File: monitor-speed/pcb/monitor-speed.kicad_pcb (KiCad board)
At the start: 2 copper layers, 60 x 70 mm, 0 parts

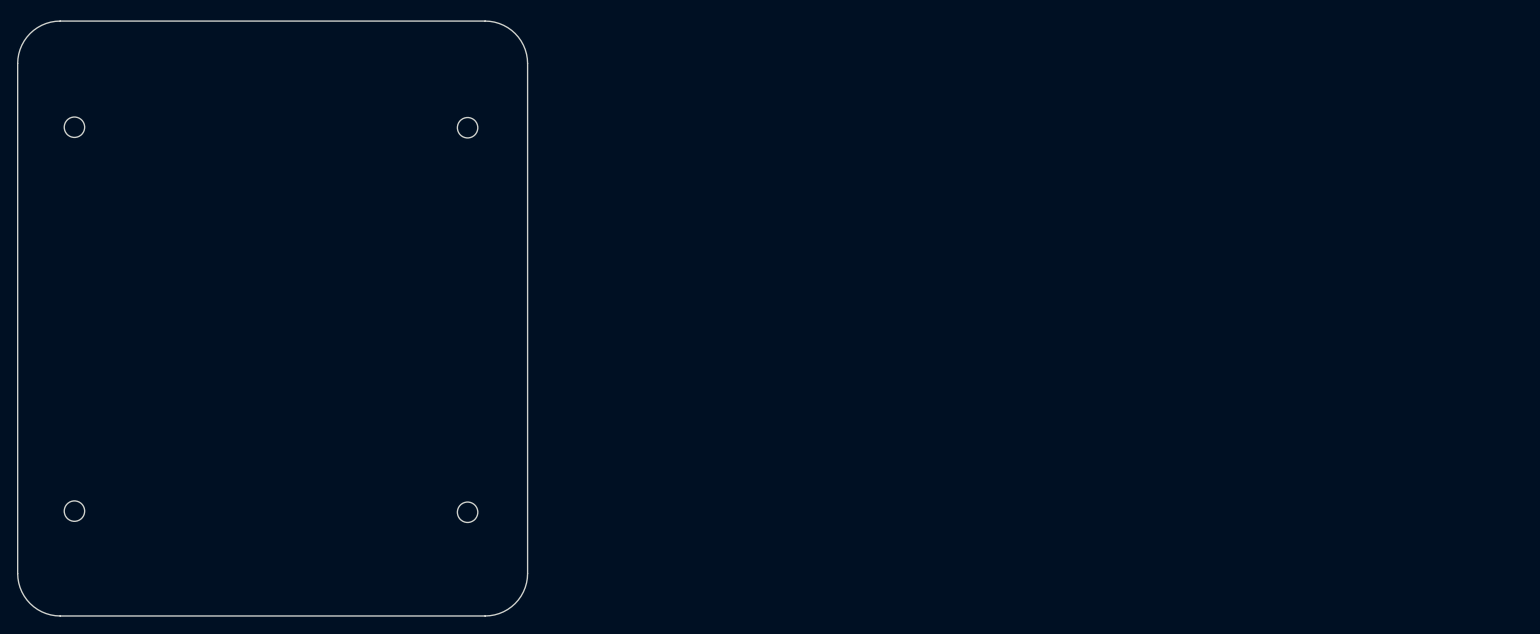
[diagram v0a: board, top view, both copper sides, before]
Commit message: Agregue capas interiores....
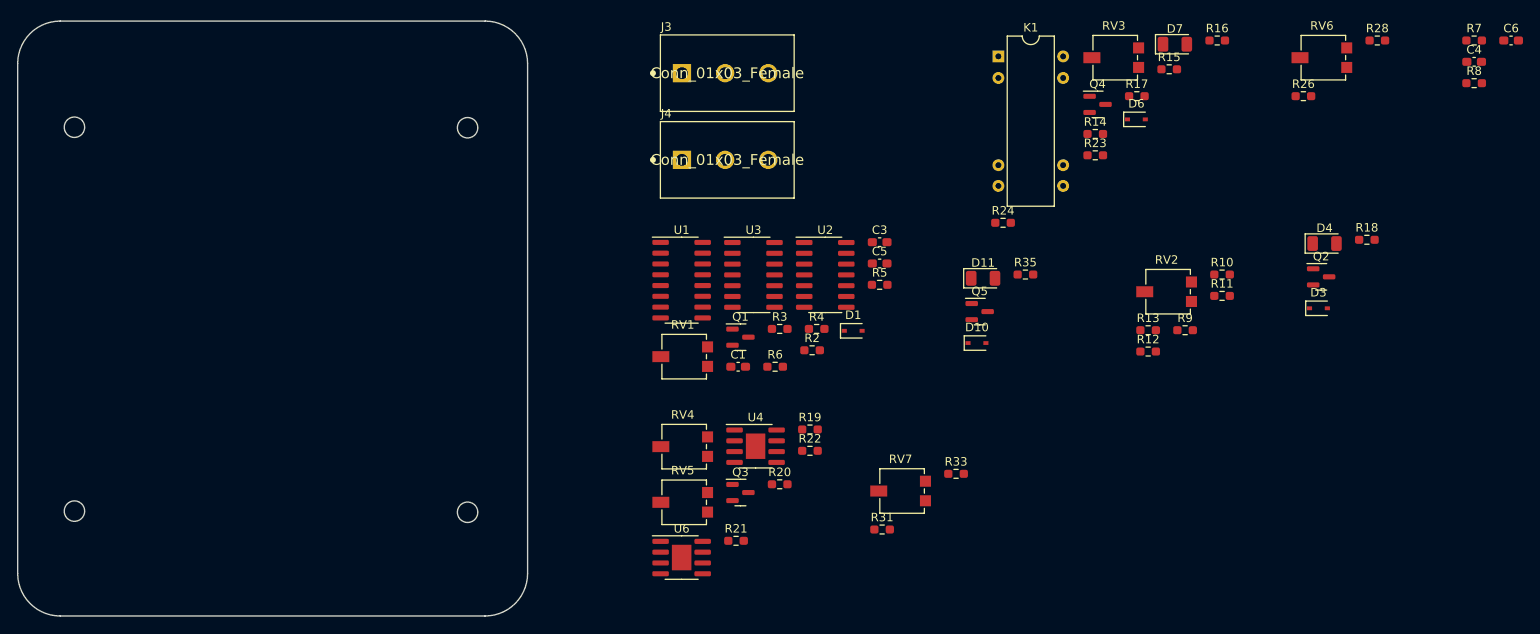
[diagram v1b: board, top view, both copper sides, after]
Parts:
- added C1: 100nF, Capacitor_SMD:C_0603_1608Metric_Pad1.08x0.95mm_HandSolder, F.Cu at (134.8, -93.3)
- added C3: 0.022uF, Capacitor_SMD:C_0603_1608Metric_Pad1.08x0.95mm_HandSolder, F.Cu at (151.4, -108.0)
- added C4: 1uF, Capacitor_SMD:C_0603_1608Metric_Pad1.08x0.95mm_HandSolder, F.Cu at (221.4, -129.2)
- added C5: 100nF, Capacitor_SMD:C_0603_1608Metric_Pad1.08x0.95mm_HandSolder, F.Cu at (151.4, -105.5)
- added C6: 1uF, Capacitor_SMD:C_0603_1608Metric_Pad1.08x0.95mm_HandSolder, F.Cu at (225.7, -131.7)
- added D1: 1N4148, Diode_SMD:D_SOD-323, F.Cu at (148.3, -97.6)
- added D10: 1N4148, Diode_SMD:D_SOD-323, F.Cu at (162.9, -96.1)
- added D11: RED, LED_SMD:LED_1206_3216Metric, F.Cu at (163.6, -103.7)
- added D3: 1N4148, Diode_SMD:D_SOD-323, F.Cu at (203.1, -100.2)
- added D4: RED, LED_SMD:LED_1206_3216Metric, F.Cu at (203.8, -107.8)
- added D6: 1N4148, Diode_SMD:D_SOD-323, F.Cu at (181.6, -122.4)
- added D7: LED, LED_SMD:LED_1206_3216Metric, F.Cu at (186.2, -131.3)
- added J3: Conn_01x03_Female, eec:TE-282841-3-0, F.Cu at (133.5, -127.9)
- added J4: Conn_01x03_Female, eec:TE-282841-3-0, F.Cu at (133.5, -117.7)
- added K1: DIPxx-1Cxx-51x, Relay_THT:Relay_StandexMeder_DIP_LowProfile, F.Cu at (165.4, -129.8)
- added Q1: BC848, Package_TO_SOT_SMD:SOT-23, F.Cu at (135.0, -96.8)
- added Q2: BC848, Package_TO_SOT_SMD:SOT-23, F.Cu at (203.4, -103.9)
- added Q3: PN2222A, Package_TO_SOT_SMD:SOT-23, F.Cu at (135.0, -78.5)
- added Q4: BC848, Package_TO_SOT_SMD:SOT-23, F.Cu at (177.1, -124.2)
- added Q5: BC848, Package_TO_SOT_SMD:SOT-23, F.Cu at (163.2, -99.8)
- added R10: 10M, Resistor_SMD:R_0603_1608Metric_Pad0.98x0.95mm_HandSolder, F.Cu at (191.7, -104.2)
- added R11: 47K, Resistor_SMD:R_0603_1608Metric_Pad0.98x0.95mm_HandSolder, F.Cu at (191.7, -101.7)
- added R12: 68K, Resistor_SMD:R_0603_1608Metric_Pad0.98x0.95mm_HandSolder, F.Cu at (183.0, -95.1)
- added R13: 1k, Resistor_SMD:R_0603_1608Metric_Pad0.98x0.95mm_HandSolder, F.Cu at (183.0, -97.6)
- added R14: 47K, Resistor_SMD:R_0603_1608Metric_Pad0.98x0.95mm_HandSolder, F.Cu at (176.8, -120.7)
- added R15: 10K, Resistor_SMD:R_0603_1608Metric_Pad0.98x0.95mm_HandSolder, F.Cu at (185.5, -128.3)
- added R16: 68K, Resistor_SMD:R_0603_1608Metric_Pad0.98x0.95mm_HandSolder, F.Cu at (191.1, -131.7)
- added R17: 10M, Resistor_SMD:R_0603_1608Metric_Pad0.98x0.95mm_HandSolder, F.Cu at (181.7, -125.2)
- added R18: 6.8K, Resistor_SMD:R_0603_1608Metric_Pad0.98x0.95mm_HandSolder, F.Cu at (208.8, -108.3)
- added R19: 10k, Resistor_SMD:R_0603_1608Metric_Pad0.98x0.95mm_HandSolder, F.Cu at (143.2, -85.9)
- added R2: 100K, Resistor_SMD:R_0603_1608Metric_Pad0.98x0.95mm_HandSolder, F.Cu at (143.5, -95.3)
- added R20: 100k, Resistor_SMD:R_0603_1608Metric_Pad0.98x0.95mm_HandSolder, F.Cu at (139.7, -79.5)
- added R21: 1k, Resistor_SMD:R_0603_1608Metric_Pad0.98x0.95mm_HandSolder, F.Cu at (134.5, -72.8)
- added R22: 330, Resistor_SMD:R_0603_1608Metric_Pad0.98x0.95mm_HandSolder, F.Cu at (143.2, -83.4)
- added R23: 1k, Resistor_SMD:R_0603_1608Metric_Pad0.98x0.95mm_HandSolder, F.Cu at (176.8, -118.2)
- added R24: 6.8K, Resistor_SMD:R_0603_1608Metric_Pad0.98x0.95mm_HandSolder, F.Cu at (165.9, -110.3)
- added R26: 2k7, Resistor_SMD:R_0603_1608Metric_Pad0.98x0.95mm_HandSolder, F.Cu at (201.3, -125.2)
- added R28: 1k5, Resistor_SMD:R_0603_1608Metric_Pad0.98x0.95mm_HandSolder, F.Cu at (210.0, -131.7)
- added R3: 100K, Resistor_SMD:R_0603_1608Metric_Pad0.98x0.95mm_HandSolder, F.Cu at (139.7, -97.8)
- added R31: 2k7, Resistor_SMD:R_0603_1608Metric_Pad0.98x0.95mm_HandSolder, F.Cu at (151.7, -74.2)
- added R33: 1k5, Resistor_SMD:R_0603_1608Metric_Pad0.98x0.95mm_HandSolder, F.Cu at (160.4, -80.7)
- added R35: 6.8K, Resistor_SMD:R_0603_1608Metric_Pad0.98x0.95mm_HandSolder, F.Cu at (168.6, -104.2)
- added R4: 100K, Resistor_SMD:R_0603_1608Metric_Pad0.98x0.95mm_HandSolder, F.Cu at (144.0, -97.8)
- added R5: 100K, Resistor_SMD:R_0603_1608Metric_Pad0.98x0.95mm_HandSolder, F.Cu at (151.4, -103.0)
- added R6: 100K, Resistor_SMD:R_0603_1608Metric_Pad0.98x0.95mm_HandSolder, F.Cu at (139.1, -93.3)
- added R7: 100K, Resistor_SMD:R_0603_1608Metric_Pad0.98x0.95mm_HandSolder, F.Cu at (221.4, -131.7)
- added R8: 100K, Resistor_SMD:R_0603_1608Metric_Pad0.98x0.95mm_HandSolder, F.Cu at (221.4, -126.7)
- added R9: 10K, Resistor_SMD:R_0603_1608Metric_Pad0.98x0.95mm_HandSolder, F.Cu at (187.4, -97.6)
- added RV1: 20K, Potentiometer_SMD:Potentiometer_Vishay_TS53YL_Vertical, F.Cu at (128.4, -94.5)
- added RV2: 10K, Potentiometer_SMD:Potentiometer_Vishay_TS53YL_Vertical, F.Cu at (185.4, -102.2)
- added RV3: 10K, Potentiometer_SMD:Potentiometer_Vishay_TS53YL_Vertical, F.Cu at (179.1, -129.7)
- added RV4: 10k, Potentiometer_SMD:Potentiometer_Vishay_TS53YL_Vertical, F.Cu at (128.4, -83.9)
- added RV5: 10k, Potentiometer_SMD:Potentiometer_Vishay_TS53YL_Vertical, F.Cu at (128.4, -77.4)
- added RV6: 10K, Potentiometer_SMD:Potentiometer_Vishay_TS53YL_Vertical, F.Cu at (203.6, -129.7)
- added RV7: 10K, Potentiometer_SMD:Potentiometer_Vishay_TS53YL_Vertical, F.Cu at (154.1, -78.7)
- added U1: 4040, Package_SO:SOIC-16_3.9x9.9mm_P1.27mm, F.Cu at (128.1, -103.5)
- added U2: 4070, Package_SO:SOIC-14_3.9x8.7mm_P1.27mm, F.Cu at (145.0, -104.1)
- added U3: 4070, Package_SO:SOIC-14_3.9x8.7mm_P1.27mm, F.Cu at (136.6, -104.1)
- added U4: TL082, Package_SO:SOIC-8-1EP_3.9x4.9mm_P1.27mm_EP2.29x3mm, F.Cu at (136.8, -84.0)
- added U6: TL082, Package_SO:SOIC-8-1EP_3.9x4.9mm_P1.27mm_EP2.29x3mm, F.Cu at (128.1, -70.9)
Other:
- copper layers 2 -> 4
